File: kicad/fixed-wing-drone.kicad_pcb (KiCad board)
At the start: 2 copper layers, 95 x 61.5 mm, 29 parts, among them J1 1, J10 ACC POWER, J11 RC POWER, J12 Airspeed I2C, J13 EXTRA STEMMA QT, J14 QT I2C, J15 QT I2C, J17 FC UBEC Input, J18 ESC UBEC Input, J19 Secondary ESC, J2 2, J20 LIDAR BKUP, J21 AUX, J3 3, J4 4, J5 5, J6 6, J7 RC SIGNAL IN, J8 LIDAR, J9 GPS, Q1 FC REV POLARITY PROT, Q2 ESC REV POLARITY PROT, U1 ESP32-S3-DevKitC

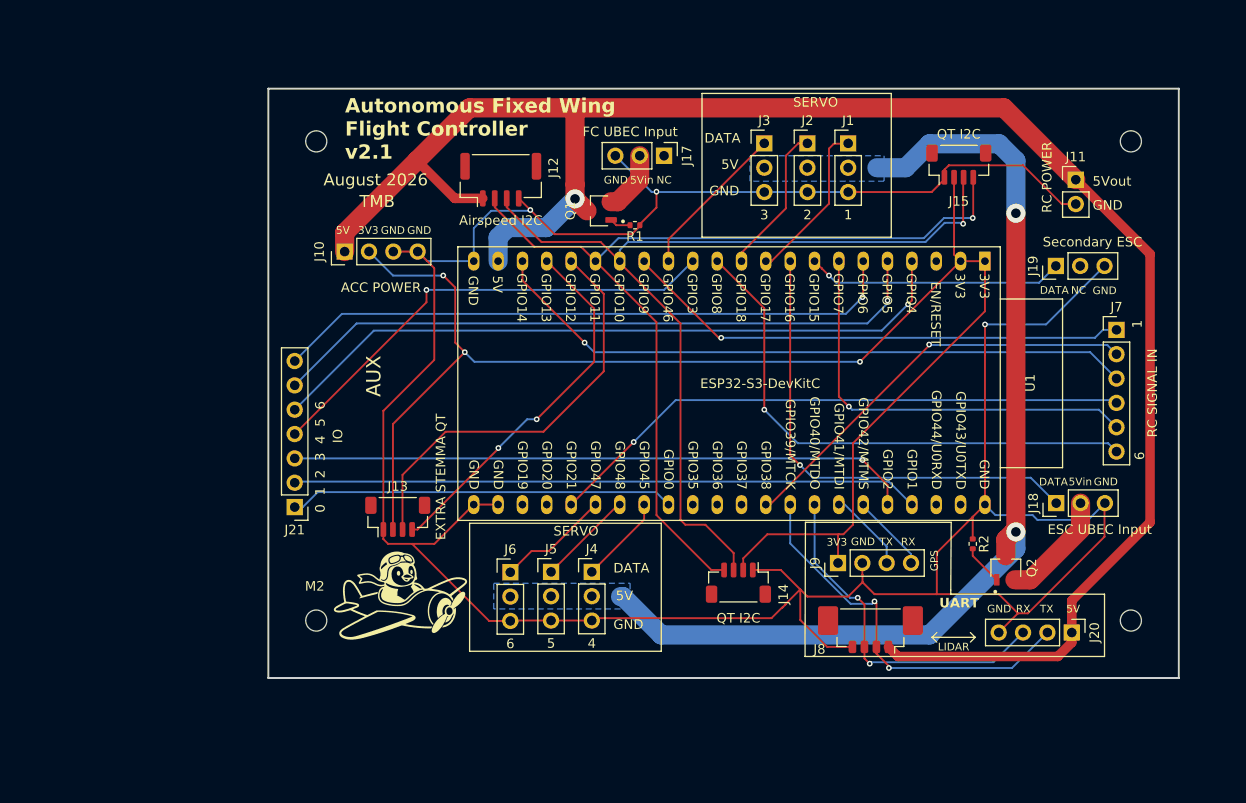
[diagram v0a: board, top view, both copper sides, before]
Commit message: PCB v3.0
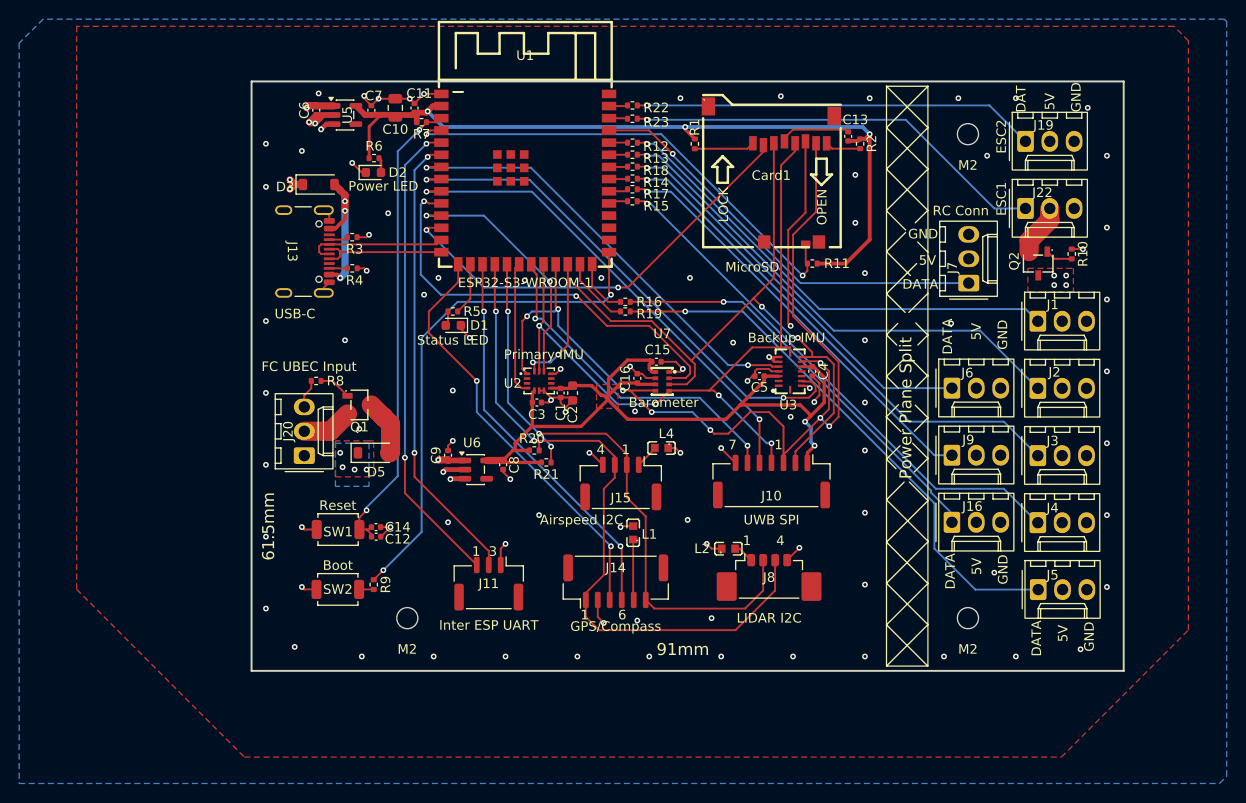
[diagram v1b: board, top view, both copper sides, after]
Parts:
- removed J12: Airspeed I2C, Connector_JST:JST_GH_BM04B-GHS-TBT_1x04-1MP_P1.25mm_Vertical
- removed J17: FC UBEC Input, Connector_PinHeader_2.54mm:PinHeader_1x03_P2.54mm_Vertical
- removed J18: ESC UBEC Input, Connector_PinHeader_2.54mm:PinHeader_1x03_P2.54mm_Vertical
- removed J21: AUX, Connector_PinHeader_2.54mm:PinHeader_1x07_P2.54mm_Vertical
- removed REF** (x4): MountingHole_2.2mm_M2, MountingHole:MountingHole_2.2mm_M2
- added C1: 100nF, Capacitor_SMD:C_0402_1005Metric, F.Cu at (130.5, 94.8)
- added C10: 22uF, Capacitor_SMD:C_0805_2012Metric, F.Cu at (113.2, 65.0)
- added C11: 100nF, Capacitor_SMD:C_0402_1005Metric, F.Cu at (115.2, 65.0)
- added C12: 1uF, Capacitor_SMD:C_0402_1005Metric, F.Cu at (111.2, 109.8)
- added C13: 100nF, Capacitor_SMD:C_0402_1005Metric, F.Cu at (160.5, 68.0)
- added C14: 100nF, Capacitor_SMD:C_0402_1005Metric, F.Cu at (111.2, 108.8)
- added C15: 100nF, Capacitor_SMD:C_0402_1005Metric, F.Cu at (140.5, 91.5)
- added C16: 100nF, Capacitor_SMD:C_0402_1005Metric, F.Cu at (138.5, 93.2)
- added C2: 2.2 uF, Capacitor_SMD:C_0603_1608Metric, F.Cu at (131.8, 94.8)
- added C3: 10 nF, Capacitor_SMD:C_0402_1005Metric, F.Cu at (128.0, 95.8)
- added C4: 100nF, Capacitor_SMD:C_0402_1005Metric, F.Cu at (156.8, 92.5)
- added C5: 100nF, Capacitor_SMD:C_0402_1005Metric, F.Cu at (151.2, 93.0)
- added C6: 1uF, Capacitor_SMD:C_0402_1005Metric, F.Cu at (105.0, 65.2)
- added C7: 1uF, Capacitor_SMD:C_0402_1005Metric, F.Cu at (110.8, 65.2)
- added C8: 1uF, Capacitor_SMD:C_0402_1005Metric, F.Cu at (124.5, 102.2)
- added C9: 1uF, Capacitor_SMD:C_0402_1005Metric, F.Cu at (118.8, 101.2)
- added Card1: MicroSD, easyeda2kicad:TF-SMD_XKTF-001B, F.Cu at (152.5, 72.1)
- added D1: Status LED, LED_SMD:LED_0603_1608Metric, F.Cu at (119.3, 87.7)
- added D2: Power LED, LED_SMD:LED_0603_1608Metric, F.Cu at (111.0, 71.8)
- added D3: B5819W, Diode_SMD:D_SOD-123, F.Cu at (105.2, 73.0)
- added D5: B5819W, Diode_SMD:D_SOD-123, F.Cu at (111.0, 101.0)
- added J16: 8, Connector_Molex:Molex_KK-254_AE-6410-03A_1x03_P2.54mm_Vertical, F.Cu at (171.3, 108.2)
- added J22: ESC1, Connector_Molex:Molex_KK-254_AE-6410-03A_1x03_P2.54mm_Vertical, F.Cu at (179.0, 75.5)
- added L1: Ferrite Bead, easyeda2kicad:L0603, F.Cu at (138.1, 109.3)
- added L2: Ferrite Bead, easyeda2kicad:L0603, F.Cu at (148.0, 111.0)
- added L4: Ferrite Bead, easyeda2kicad:L0603, F.Cu at (141.0, 100.5)
- added M2: MountingHole_2.2mm_M2, MountingHole:MountingHole_2.2mm_M2, F.Cu at (114.5, 118.2)
- added M2: MountingHole_2.2mm_M2, MountingHole:MountingHole_2.2mm_M2, F.Cu at (173.0, 67.8)
- added M2: MountingHole_2.2mm_M2, MountingHole:MountingHole_2.2mm_M2, F.Cu at (173.0, 118.2)
- added R10: 100K, Resistor_SMD:R_0402_1005Metric, F.Cu at (183.8, 80.2)
- added R11: 10K, Resistor_SMD:R_0402_1005Metric, F.Cu at (156.8, 81.2)
- added R12: 330R, Resistor_SMD:R_0402_1005Metric, F.Cu at (138.0, 68.6)
- added R13: 330R, Resistor_SMD:R_0402_1005Metric, F.Cu at (138.0, 69.9)
- added R14: 330R, Resistor_SMD:R_0402_1005Metric, F.Cu at (138.0, 72.4)
- added R15: 330R, Resistor_SMD:R_0402_1005Metric, F.Cu at (138.0, 74.8)
- added R16: 330R, Resistor_SMD:R_0402_1005Metric, F.Cu at (137.2, 85.2)
- added R17: 330R, Resistor_SMD:R_0402_1005Metric, F.Cu at (138.0, 73.5)
- added R18: 330R, Resistor_SMD:R_0402_1005Metric, F.Cu at (138.0, 71.1)
- added R19: 330R, Resistor_SMD:R_0402_1005Metric, F.Cu at (137.2, 86.2)
- added R20: 6.8K, Resistor_SMD:R_0402_1005Metric, F.Cu at (127.8, 100.8)
- added R21: 6.8K, Resistor_SMD:R_0402_1005Metric, F.Cu at (129.0, 102.0)
- added R22: 330R, Resistor_SMD:R_0402_1005Metric, F.Cu at (138.0, 64.8)
- added R23: 330R, Resistor_SMD:R_0402_1005Metric, F.Cu at (138.0, 66.1)
- added R3: 5.1K, Resistor_SMD:R_0402_1005Metric, F.Cu at (108.8, 78.5)
- added R4: 5.1K, Resistor_SMD:R_0402_1005Metric, F.Cu at (108.8, 81.8)
- added R5: 220R, Resistor_SMD:R_0402_1005Metric, F.Cu at (119.2, 86.2)
- added R6: 220R, Resistor_SMD:R_0402_1005Metric, F.Cu at (111.0, 70.2)
- added R7: 10k, Resistor_SMD:R_0402_1005Metric, F.Cu at (116.0, 66.5)
- added R8: 100K, Resistor_SMD:R_0402_1005Metric, F.Cu at (105.0, 93.5)
- added R9: 100R, Resistor_SMD:R_0402_1005Metric, F.Cu at (111.0, 114.8)
- added SW1: TS-1088, Button_Switch_SMD:SW_SPST_TS-1088-xR020, F.Cu at (107.3, 109.0)
- added SW2: TS-1088, Button_Switch_SMD:SW_SPST_TS-1088-xR020, F.Cu at (107.2, 115.2)
- added U2: Primary IMU, easyeda2kicad:LGA-14_L3.0-W2.5-P0.50-TL, F.Cu at (128.3, 93.5)
- added U3: Backup IMU, easyeda2kicad:LGA-16_L4.5-W3.0-P0.50-BL, F.Cu at (154.4, 92.5)
- added U5: AP2112K-3.3, Package_TO_SOT_SMD:SOT-23-5, F.Cu at (108.0, 65.8)
- added U6: AP2112K-3.3, Package_TO_SOT_SMD:SOT-23-5, F.Cu at (121.6, 102.8)
- added U7: Barometer, easyeda2kicad:LGA-8_L2.5-W2.0-P0.65-TR_DPS368, F.Cu at (141.1, 93.5)
- J1, J2, J3, J4, J5, J6: footprint Connector_PinHeader_2.54mm:PinHeader_1x03_P2.54mm_Vertical -> Connector_Molex:Molex_KK-254_AE-6410-03A_1x03_P2.54mm_Vertical
- J10: value ACC POWER -> UWB SPI; footprint Connector_PinHeader_2.54mm:PinHeader_1x04_P2.54mm_Vertical -> Connector_JST:JST_GH_BM07B-GHS-TBT_1x07-1MP_P1.25mm_Vertical
- J11: value RC POWER -> Inter ESP UART; footprint Connector_PinHeader_2.54mm:PinHeader_1x02_P2.54mm_Vertical -> Connector_JST:JST_GH_BM03B-GHS-TBT_1x03-1MP_P1.25mm_Vertical
- J13: value EXTRA STEMMA QT -> USB-C; footprint Connector_JST:JST_SH_BM04B-SRSS-TB_1x04-1MP_P1.00mm_Vertical -> Connector_USB:USB_C_Receptacle_GCT_USB4105-xx-A_16P_TopMnt_Horizontal
- J14: value QT I2C -> GPS/Compass; footprint Connector_JST:JST_SH_BM04B-SRSS-TB_1x04-1MP_P1.00mm_Vertical -> Connector_JST:JST_GH_BM06B-GHS-TBT_1x06-1MP_P1.25mm_Vertical
- J15: value QT I2C -> Airspeed I2C; footprint Connector_JST:JST_SH_BM04B-SRSS-TB_1x04-1MP_P1.00mm_Vertical -> Connector_JST:JST_GH_BM04B-GHS-TBT_1x04-1MP_P1.25mm_Vertical
- J19: value Secondary ESC -> ESC2; footprint Connector_PinHeader_2.54mm:PinHeader_1x03_P2.54mm_Vertical -> Connector_Molex:Molex_KK-254_AE-6410-03A_1x03_P2.54mm_Vertical
- J20: value LIDAR BKUP -> FC UBEC Input; footprint Connector_PinHeader_2.54mm:PinHeader_1x04_P2.54mm_Vertical -> Connector_Molex:Molex_KK-254_AE-6410-03A_1x03_P2.54mm_Vertical
- J7: value RC SIGNAL IN -> RC Conn; footprint Connector_PinHeader_2.54mm:PinHeader_1x06_P2.54mm_Vertical -> Connector_Molex:Molex_KK-254_AE-6410-03A_1x03_P2.54mm_Vertical
- J8: value LIDAR -> LIDAR I2C
- J9: value GPS -> 7; footprint Connector_PinHeader_2.54mm:PinHeader_1x04_P2.54mm_Vertical -> Connector_Molex:Molex_KK-254_AE-6410-03A_1x03_P2.54mm_Vertical
- Q1: value FC REV POLARITY PROT -> reverse polarity protection; footprint AO3407A:SOT95P280X125-3N -> easyeda2kicad:SOT-23-3_L2.9-W1.6-P1.90-LS2.8-BR
- Q2: value ESC REV POLARITY PROT -> reverse polarity protection; footprint AO3407A:SOT95P280X125-3N -> easyeda2kicad:SOT-23-3_L2.9-W1.6-P1.90-LS2.8-BR
- R1, R2: value 100K -> 10K
- U1: value ESP32-S3-DevKitC -> ESP32-S3-WROOM-1; footprint PCM_Espressif:ESP32-S3-DevKitC-trav-snf2 -> easyeda2kicad:WIRELM-SMD_ESP32-S3-WROOM-1
- moved J20 82.2 mm to (103.8, 101.3), turned to 90 degrees
- moved J11 74.4 mm to (123.0, 114.7), turned to 180 degrees
- moved J5 50.9 mm to (180.3, 115.3)
- moved J10 50.6 mm to (152.5, 104.0), turned to 180 degrees
- moved J6 49.9 mm to (171.3, 94.2)
- moved U1 48.7 mm to (126.8, 72.4), turned to 0 degrees
- moved J15 48.5 mm to (136.8, 104.2), turned to 180 degrees
- moved J4 46.8 mm to (180.3, 108.3)
- moved R2 43.4 mm to (161.8, 68.8)
- moved J3 43.3 mm to (180.3, 101.3)
- moved J2 35.1 mm to (180.3, 94.3)
- moved Q1 32.2 mm to (109.5, 96.0)
- moved Q2 31.9 mm to (180.3, 81.2)
- moved J13 29.7 mm to (102.7, 80.0), turned to -90 degrees
- moved J1 27.1 mm to (180.3, 87.3)
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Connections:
- J1 pad 1: /SERVO_OUT_1 -> Net-(J1-Pin_1)
- J1 pad 2: /SERVO_5v -> /actuator_io/esc_io/SERVO_5V
- J10 pad 1: /FC_5v -> /SENSOR_3V3
- J10 pad 2: +3V3 -> /MOSI
- J10 pad 3: GND -> /MISO
- J10 pad 4: GND -> /SCK
- J11 pad 1: /FC_5v -> GND
- J11 pad 2: GND -> /INTER_ESP_TX
- J14 pad 1: GND -> /SDA
- J14 pad 2: +3V3 -> GND
- J14 pad 3: /SDA -> /GPS_RX
- J14 pad 4: /SCL -> /GPS_TX
- J15 pad 1: GND -> Net-(J15-Pin_1)
- J15 pad 2: +3V3 -> /SCL
- J15 pad 4: /SCL -> GND
- J19 pad 1: /SECONDARY_ESC_SIGNAL -> Net-(J19-Pin_1)
- J2 pad 1: /SERVO_OUT_2 -> Net-(J2-Pin_1)
- J2 pad 2: /SERVO_5v -> /actuator_io/esc_io/SERVO_5V
- J20 pad 1: /FC_5v -> unconnected-(J20-Pin_1-Pad1)
- J20 pad 2: /LIDAR_TX -> Net-(J20-Pin_2)
- J20 pad 3: /LIDAR_RX -> GND
- J3 pad 1: /SERVO_OUT_3 -> Net-(J3-Pin_1)
- J3 pad 2: /SERVO_5v -> /actuator_io/esc_io/SERVO_5V
- J4 pad 1: /SERVO_OUT_4 -> Net-(J4-Pin_1)
- J4 pad 2: /SERVO_5v -> /actuator_io/esc_io/SERVO_5V
- J5 pad 1: /SERVO_OUT_5 -> Net-(J5-Pin_1)
- J5 pad 2: /SERVO_5v -> /actuator_io/esc_io/SERVO_5V
- J6 pad 1: /SERVO_OUT_6 -> Net-(J6-Pin_1)
- J6 pad 2: /SERVO_5v -> /actuator_io/esc_io/SERVO_5V
- J7 pad 1: /RECIEVER_1 -> /RC_SBUS
- J7 pad 2: /RECIEVER_2 -> /actuator_io/esc_io/SERVO_5V
- J7 pad 3: /RECIEVER_3 -> GND
- J8 pad 1: /FC_5v -> Net-(J8-Pin_1)
- J8 pad 2: /LIDAR_TX -> /SCL
- J8 pad 3: /LIDAR_RX -> /SDA
- J9 pad 1: +3V3 -> Net-(J9-Pin_1)
- J9 pad 2: GND -> /actuator_io/esc_io/SERVO_5V
- J9 pad 3: /GPS_TX -> GND
- Q1 pad 1: Net-(Q1-Pad1) -> Net-(Q1-G)
- Q1 pad 2: Net-(J17-Pin_2) -> Net-(J20-Pin_2)
- Q1 pad 3: /FC_5v -> Net-(D5-A)
- Q2 pad 1: Net-(Q2-Pad1) -> Net-(Q2-G)
- Q2 pad 3: /SERVO_5v -> /actuator_io/esc_io/SERVO_5V
- R1 pad 1: GND -> /ESP_3V3
- R1 pad 2: Net-(Q1-Pad1) -> Net-(Card1-DAT2)
- R2 pad 1: GND -> /ESP_3V3
- R2 pad 2: Net-(Q2-Pad1) -> Net-(Card1-DAT1)
- U1 pad 1: +3V3 -> GND
- U1 pad 10: /SERVO_OUT_1 -> /BAROMETER_CS
- U1 pad 11: /SERVO_OUT_2 -> /IMU1_CS
- U1 pad 12: /RECIEVER_6 -> /SD_CS
- U1 pad 13: /ACC_3 -> /esp32s3/DATA-
- U1 pad 14: /SERVO_OUT_3 -> /esp32s3/DATA+
- U1 pad 15: /RECIEVER_1 -> /GPS_RX
- U1 pad 16: /SDA -> /STATUS_LED
- U1 pad 17: /SCL -> /GPS_TX
- U1 pad 18: /EXTRA_QT_YELLOW -> /SDA
- U1 pad 19: /EXTRA_QT_BLUE -> /SCL
- U1 pad 2: +3V3 -> /ESP_3V3
- U1 pad 20: /RECIEVER_3 -> /IMU1_INT
- U1 pad 21: /FC_5v -> /UWB_INT
- U1 pad 22: GND -> /SCK
- U1 pad 23: GND -> /MISO
- U1 pad 24: GND -> /MOSI
- U1 pad 25: unconnected-(U1-GPIO19/USB_D--Pad25) -> /SERVO_OUT5
- U1 pad 26: unconnected-(U1-GPIO20/USB_D+-Pad26) -> /SERVO_OUT8
- U1 pad 27: /RECIEVER_4 -> /esp32s3/BOOT
- U1 pad 28: /SERVO_OUT_6 -> unconnected-(U1-IO35-Pad28)
- U1 pad 29: /SERVO_OUT_5 -> unconnected-(U1-IO36-Pad29)
- U1 pad 3: unconnected-(U1-CHIP_PU-Pad3) -> /esp32s3/EN
- U1 pad 30: /SERVO_OUT_4 -> unconnected-(U1-IO37-Pad30)
- U1 pad 31: /ACC_0 -> /SERVO_OUT4
- U1 pad 32: unconnected-(U1-GPIO35-Pad32) -> /SERVO_OUT7
- U1 pad 33: unconnected-(U1-GPIO36-Pad33) -> /SERVO_OUT3
- U1 pad 34: unconnected-(U1-GPIO37-Pad34) -> /SERVO_OUT6
- U1 pad 35: /RECIEVER_2 -> /SERVO_OUT2
- U1 pad 36: /LIDAR_TX -> /SERVO_OUT1
- U1 pad 37: /LIDAR_RX -> /RC_SBUS
- U1 pad 38: /GPS_TX -> /ESC_OUT1
- U1 pad 39: /GPS_RX -> /ESC_OUT2
- U1 pad 4: /ACC_4 -> /SD_CARD_DETECT
- U1 pad 40: /ACC_2 -> GND
- U1 pad 41: /ACC_1 -> GND
- U1 pad 5: /ACC_5 -> /INTER_ESP_RX
- U1 pad 6: /ACC_6 -> /INTER_ESP_TX
- U1 pad 7: /RECIEVER_5 -> /IMU2_GYRO_CS
- U1 pad 8: /SECONDARY_ESC_SIGNAL -> /IMU2_ACCEL_CS
- U1 pad 9: /PRIMARY_ESC_SIGNAL -> /UWB_CS
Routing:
- net GND: track 305.8 -> 96.1 mm, vias 3 -> 93
- net /FC_5v: track 193.7 -> 0.00 mm, vias 1 -> 0
- net +3V3: track 158.5 -> 0.00 mm, vias 3 -> 0
- net /SERVO_5v: track 106.5 -> 0.00 mm, vias 2 -> 0
- net /MISO: track 0.00 -> 105.7 mm, vias 0 -> 9
- net /SENSOR_3V3: track 0.00 -> 88.4 mm, vias 0 -> 2
- net /MOSI: track 0.00 -> 86.0 mm, vias 0 -> 4
- net /ESP_3V3: track 0.00 -> 84.7 mm, vias 0 -> 3
- net /SCK: track 0.00 -> 76.7 mm, vias 0 -> 4
- net /ACC_4: track 73.2 -> 0.00 mm, vias 1 -> 0
- net /ACC_5: track 69.9 -> 0.00 mm, vias 1 -> 0
- net /RECIEVER_3: track 68.2 -> 0.00 mm, vias 1 -> 0
- net /ACC_6: track 65.8 -> 0.00 mm, vias 1 -> 0
- net /ACC_1: track 65.4 -> 0.00 mm
- net /ACC_2: track 65.1 -> 0.00 mm, vias 1 -> 0
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- added copper zone on B.Cu, net /FC_5V
- added copper zone on F.Cu, net /FC_5V
- added copper zone on In2.Cu, net /FC_5V
- added copper zone on F.Cu, net /SENSOR_3V3
- added copper zone on F.Cu, net /actuator_io/esc_io/SERVO_5V
- added copper zone on In2.Cu, net /actuator_io/esc_io/SERVO_5V
- added copper zone on B.Cu, net GND
- added copper zone on F.Cu, net GND
- added copper zone on In1.Cu, net GND
- removed copper zone on B.Cu, net /SERVO_5v
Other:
- board size 95 x 61.5 mm -> 91 x 61.5 mm
- copper layers 2 -> 4
- board text added: "1 3"
- board text added: "1 4"
- board text added: "1 6"
- board text added: "4 1"
- board text added: "61.5mm"
- board text added: "7 1"
- board text added: "91mm"
- board text added: "Autonomous Fixed Wing Flight Controller v3.0"
- board text added: "C9"
- board text added: "DAT"
- board text added: "Power Plane Split"
- board text added: "September 2026"
- board text removed: "0 1 2 3 4 5 6"
- board text removed: "1"
- board text removed: "3V3"
- board text removed: "5Vin"
- board text removed: "5Vout"
- board text removed: "6"
- board text removed: "August 2026"
- board text removed: "Autonomous Fixed Wing Flight Controller v2.1"
- board text removed: "GPS"
- board text removed: "IO"
- board text removed: "LIDAR"
- board text removed: "M2"
- board text removed: "NC"
- board text removed: "RX"
- board text removed: "SERVO"
- board text removed: "TX"
- board text removed: "UART"
